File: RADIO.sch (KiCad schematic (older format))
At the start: 20 parts, among them U801 A7, U802 SIM_SLOT

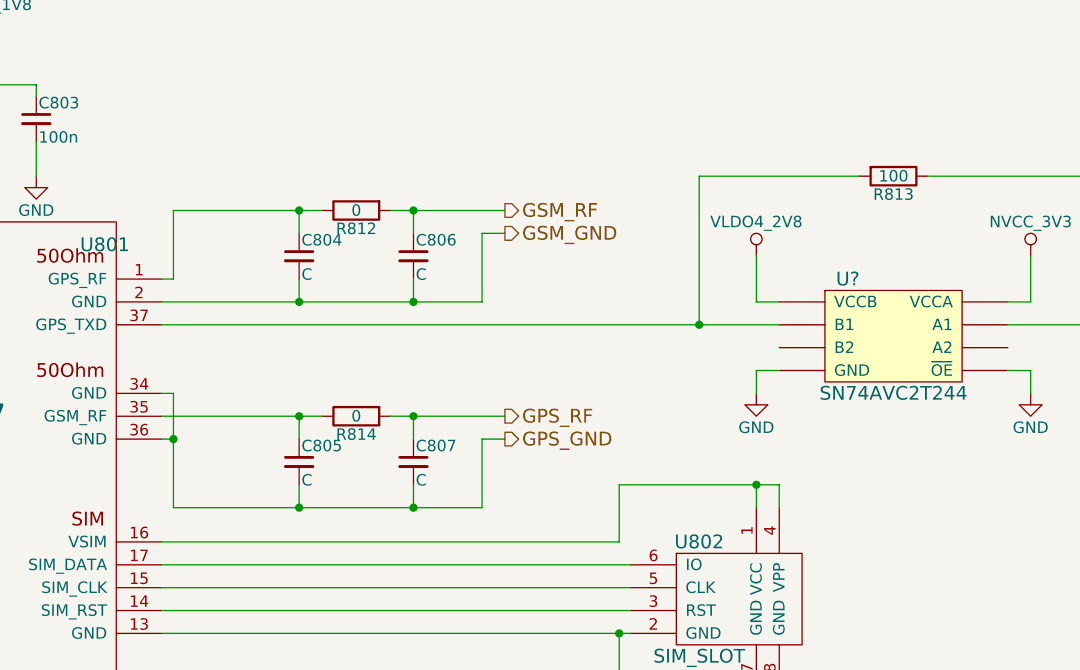
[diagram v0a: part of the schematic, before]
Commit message: modified adui circuit
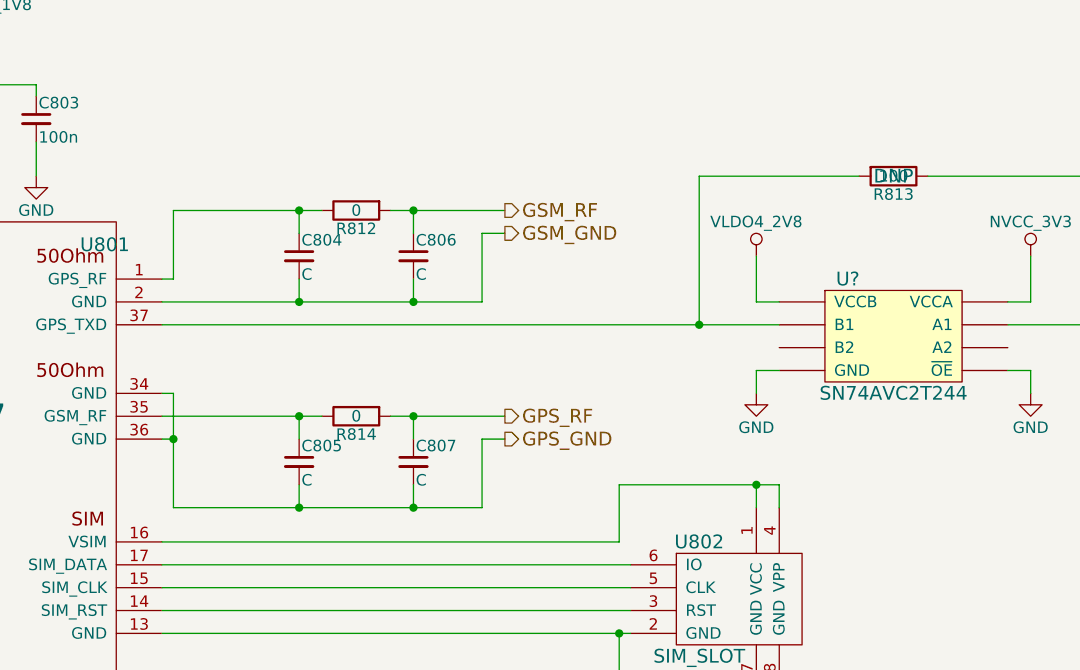
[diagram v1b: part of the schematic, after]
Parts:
- R813: manufacture (none) -> DNP
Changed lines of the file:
@@
 LIBS:mtfc8gacaeam-1m_wt
 LIBS:sn74avc2t244
-LIBS:lsm9ds1
+LIBS:WM8960CGEFL
 LIBS:3210retro-cache
 EELAYER 25 0
@@
 	12050 4000 11950 4000
 Wire Wire Line
-	11950 4300 11950 4000
+	11950 4000 11950 4300
 Wire Wire Line
 	10600 3800 10600 4300
@@
 	12050 3100 11950 3100
 Wire Wire Line
-	11950 3400 11950 3100
-Wire Wire Line
-	10550 3400 11950 3400
+	11950 3100 11950 3400
+Wire Wire Line
+	11950 3400 10550 3400
 Wire Wire Line
 	11150 3300 11150 3400
@@
 F 2 "Resistors_SMD:R_0603" V 13680 2850 50  0001 C CNN
 F 3 "" H 13750 2850 50  0000 C CNN
+F 4 "DNP" V 13750 2850 60  0000 C CNN "manufacture"
 	1    13750 2850
 	0    1    1    0
